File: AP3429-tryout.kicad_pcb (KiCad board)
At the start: 2 copper layers, 90 x 75 mm, 61 parts, among them J1 Conn_01x05, J2 Conn_01x02, U1 AP3429, U10 AMS1117-3.3, U2 AP3429, U3 AP3429, U4 AP2120N, U5 AMS1117-3.3, U6 AMS1117-3.3, U7 AMS1117-3.3, U8 AMS1117-3.3, U9 AMS1117-3.3

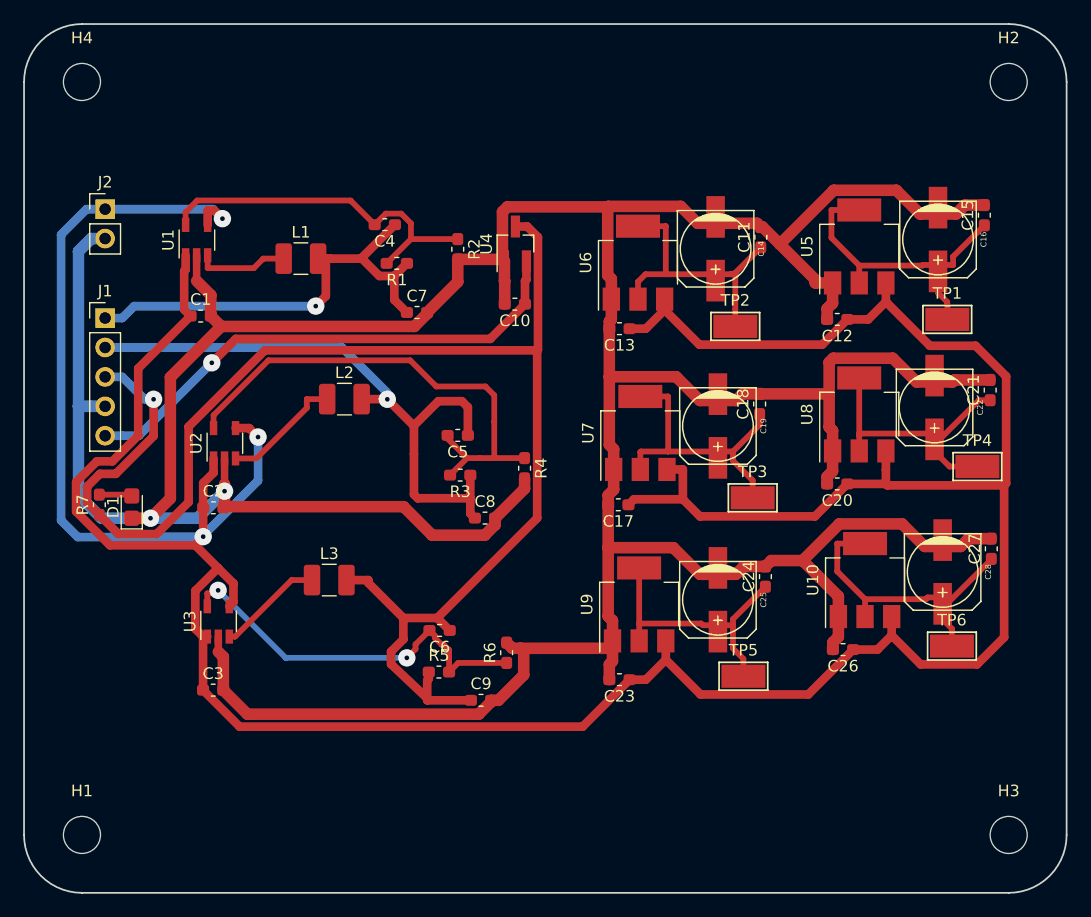
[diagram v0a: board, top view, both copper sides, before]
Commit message: update,
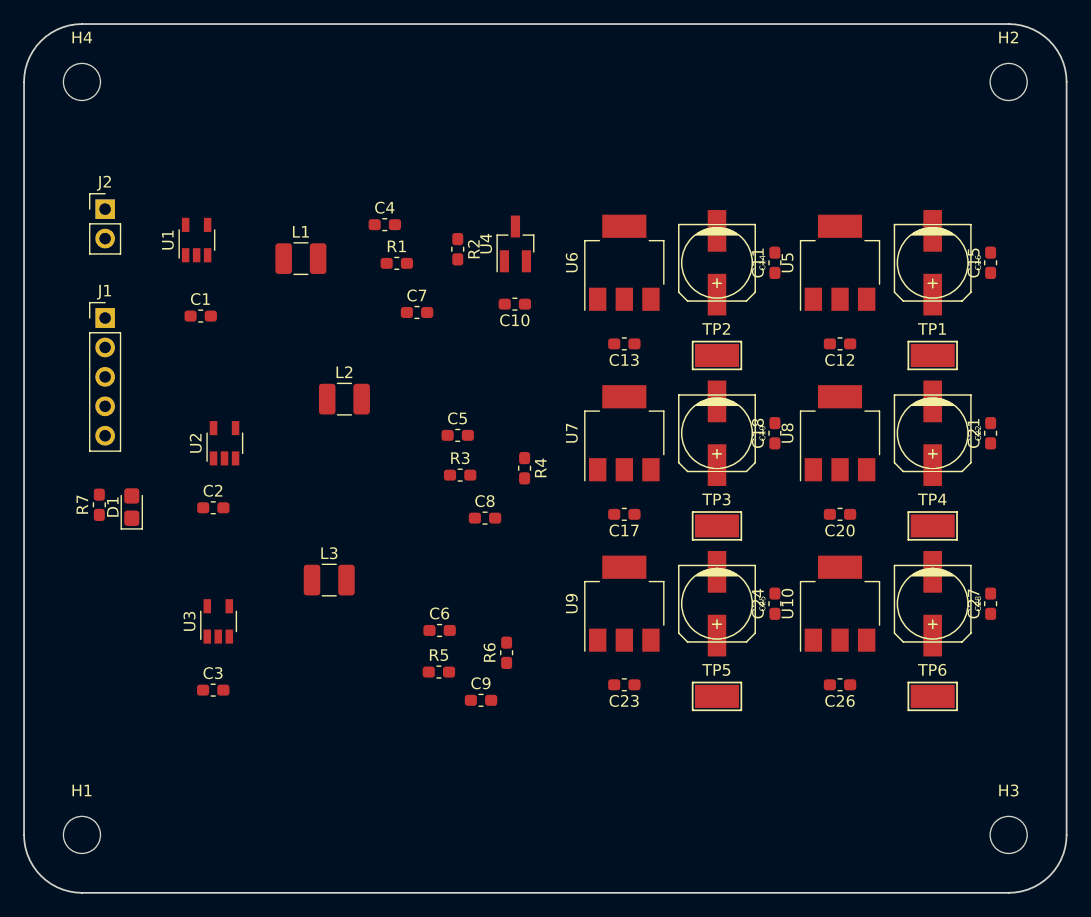
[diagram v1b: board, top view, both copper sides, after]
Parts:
- moved TP4 6.42 mm to (78.4, 43.3)
- moved C27 4.74 mm to (83.4, 50.0)
- moved TP6 4.65 mm to (78.4, 58.0)
- moved C15 4.15 mm to (83.4, 20.6)
- moved TP3 3.92 mm to (59.8, 43.3)
- moved C21 3.73 mm to (83.4, 35.3)
- moved TP1 3.36 mm to (78.4, 28.6)
- moved C26 3.05 mm to (70.4, 57.0)
- moved U10 2.97 mm to (70.4, 50.0)
- moved TP2 2.97 mm to (59.8, 28.6)
- moved C28 2.87 mm to (78.4, 50.0)
- moved TP5 2.87 mm to (59.8, 58.0)
- moved C18 2.85 mm to (64.8, 35.3)
- moved C20 2.64 mm to (70.4, 42.3)
- moved C11 2.52 mm to (64.8, 20.6)
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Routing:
- net GND: track 372.4 -> 0.00 mm, vias 2 -> 0
- net +5V: track 320.6 -> 0.00 mm, vias 3 -> 0
- net +3V3: track 131.8 -> 0.00 mm, vias 1 -> 0
- net +1V8: track 54.7 -> 0.00 mm, vias 1 -> 0
- net +3V0: track 44.7 -> 0.00 mm, vias 1 -> 0
- net Net-(C5-Pad2): track 43.7 -> 0.00 mm
- net +1V2: track 39.3 -> 0.00 mm, vias 1 -> 0
- net Net-(C6-Pad2): track 33.7 -> 0.00 mm, vias 2 -> 0
- net Net-(C4-Pad2): track 30.9 -> 0.00 mm
- net Net-(C15-Pad1): track 27.4 -> 0.00 mm
- net Net-(C27-Pad1): track 27.0 -> 0.00 mm
- net Net-(C18-Pad1): track 25.6 -> 0.00 mm
- net Net-(C21-Pad1): track 25.4 -> 0.00 mm
- net Net-(C11-Pad1): track 24.5 -> 0.00 mm
- net Net-(C24-Pad1): track 23.7 -> 0.00 mm
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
